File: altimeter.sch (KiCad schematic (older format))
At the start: 43 parts, among them Q101 DMG2301L, Q102 NTR4003NT1G, Q103 SISS05dn, U1 LMV331, U101 STM32F303CCTx, U102 S25FL512SAGMFIR11, U103 AIS2120SXTR, U104 MIC5219-3.3YM5, U105 LF50_TO252, U106 BMI088, U107 MS5611-01BA, Y1 Crystal_GND24

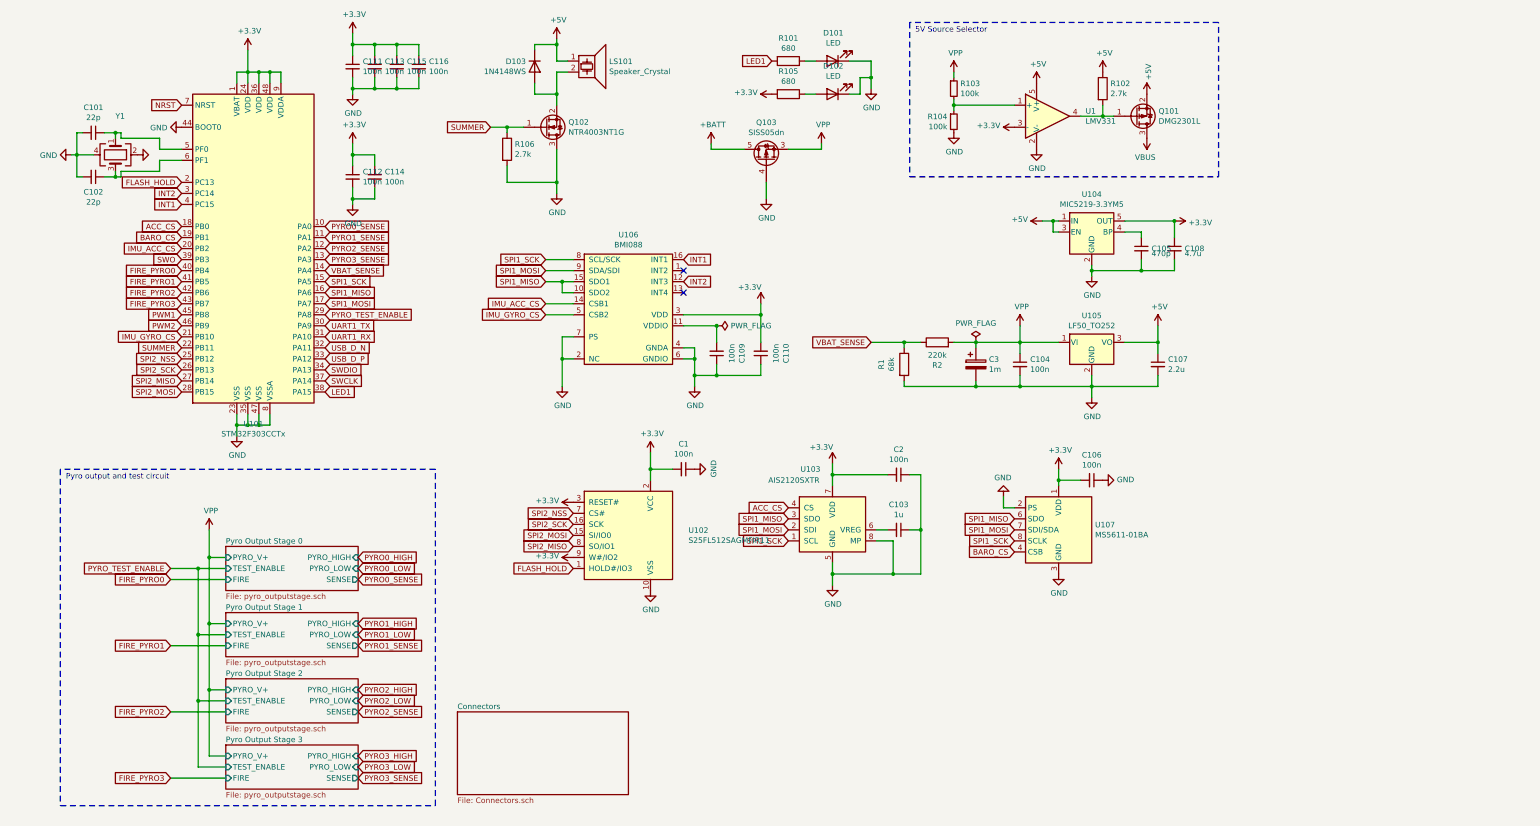
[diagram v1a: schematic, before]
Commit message: v1.2 rev A
Signed-off-by: Thomas Schmid <tom@binary-kitchen.de>
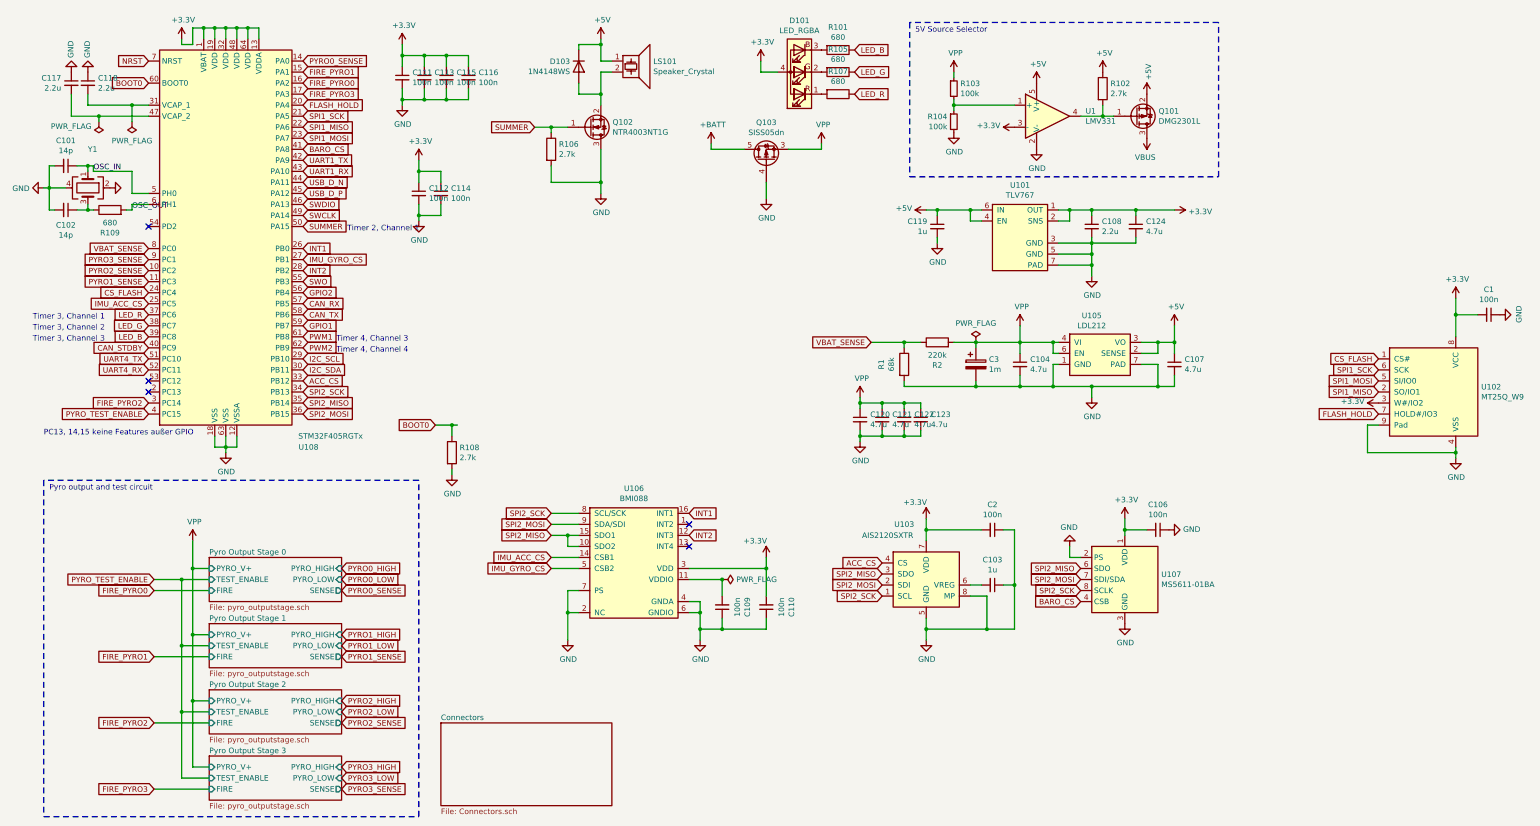
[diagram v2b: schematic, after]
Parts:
- removed C105: 470p, Capacitor_SMD:C_0603_1608Metric_Pad1.05x0.95mm_HandSolder, symbol Device:C_Small
- removed D101, D102: LED, LED_SMD:LED_0603_1608Metric, symbol Device:LED
- removed U101: STM32F303CCTx, Package_QFP:LQFP-48_7x7mm_P0.5mm, symbol MCU_ST_STM32F3:STM32F303CCTx
- removed U102: S25FL512SAGMFIR11, Package_SO:SOIC-16W_7.5x10.3mm_P1.27mm, symbol altimeter:S25L512S
- removed U104: MIC5219-3.3YM5, Package_TO_SOT_SMD:SOT-23-5, symbol Regulator_Linear:MIC5219-3.3YM5
- removed U105: LF50_TO252, Package_TO_SOT_SMD:TO-252-2, symbol Regulator_Linear:LF50_TO252
- added C117, C118: 2.2u, Capacitor_SMD:C_0402_1005Metric, symbol Device:C_Small
- added C119: 1u, Capacitor_SMD:C_0805_2012Metric, symbol Device:C_Small
- added C120, C121, C122, C123: 4.7u, Capacitor_SMD:C_0805_2012Metric_Pad1.15x1.40mm_HandSolder, symbol Device:C_Small
- added C124: 4.7u, Capacitor_SMD:C_0603_1608Metric_Pad1.05x0.95mm_HandSolder, symbol Device:C_Small
- added D101: LED_RGBA, altimeter:SMD_RGB_LED, symbol Device:LED_RGBA
- added R107, R109: 680, Resistor_SMD:R_0402_1005Metric, symbol Device:R
- added R108: 2.7k, Resistor_SMD:R_0402_1005Metric, symbol Device:R
- added U101: TLV767, altimeter:TI_WSON_TLV767, symbol altimeter:TLV767
- added U102: MT25Q_W9, altimeter:micron-wpdfn_8x6mm, symbol altimeter:MT25Q_W9
- added U105: LDL212, Package_DFN_QFN:DFN-6-1EP_3x3mm_P0.95mm_EP1.7x2.6mm, symbol altimeter:LDL212
- added U108: STM32F405RGTx, Package_QFP:LQFP-64_10x10mm_P0.5mm, symbol MCU_ST_STM32F4:STM32F405RGTx
- C101, C102: value 22p -> 14p
- C104: value 100n -> 4.7u
- C107: value 2.2u -> 4.7u; footprint Capacitor_SMD:C_0603_1608Metric_Pad1.05x0.95mm_HandSolder -> Capacitor_SMD:C_0805_2012Metric
- C108: value 4.7u -> 2.2u
- R106: Mouser_Link (none) -> https://www.mouser.de/ProductDetail/Vishay-Dale/CRCW04022K7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; Parnumber (none) -> CRCW04022K70FKEDC
- U1: footprint Package_TO_SOT_SMD:SOT-23-5 -> Package_TO_SOT_SMD:SOT-353_SC-70-5; Mouser_Link https://www.mouser.de/ProductDetail/ON-Semiconductor/LMV331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 -> https://www.mouser.de/datasheet/2/115/LMV331_393-335820.pdf; Parnumber LMV331SN3T1G -> LMV331SE-7
- Y1: footprint Crystal:Crystal_SMD_2520-4Pin_2.5x2.0mm -> Crystal:Crystal_SMD_2016-4Pin_2.0x1.6mm; Mouser_Link https://www.mouser.de/ProductDetail/Epson-Timing/TSX-3225-2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 -> https://www.mouser.de/ProductDetail/ECS/ECS-160-12-37B-CTN-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; Parnumber TSX-3225 24.0000MF15X-AC3 -> ECS-160-12-37B-CTN-TR
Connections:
- net +3V3: now also C124.1, D101.4 (A), U101.1 (OUT), U101.2 (SNS), U102.3 (W#/IO2), U102.8 (VCC), U108.1 (VBAT), U108.13 (VDDA), U108.19 (VDD), U108.32 (VDD), U108.48 (VDD), U108.64 (VDD); no longer R105.2
- net +5V: now also C119.1, U101.4 (EN), U101.6 (IN), U105.2 (SENSE), U105.3 (VO)
- net ACC_CS: now also U108.33 (PB12)
- net BARO_CS: now also U108.41 (PA8)
- net FIRE_PYRO0: now also U108.16 (PA2)
- net FIRE_PYRO1: now also U108.15 (PA1)
- net FIRE_PYRO2: now also U108.3 (PC14)
- net FIRE_PYRO3: now also U108.17 (PA3)
- net FLASH_HOLD: now also U102.7 (HOLD#/IO3), U108.20 (PA4)
- net GND: now also C117.1, C118.1, C119.2, C120.2, C121.2, C122.2, C123.2, C124.2, R108.2, U101.3 (GND), U101.5 (GND), U101.7 (PAD), U102.4 (VSS), U102.9 (Pad), U105.1 (GND), U105.7 (PAD), U108.12 (VSSA), U108.18 (VSS), U108.63 (VSS)
- net IMU_ACC_CS: now also U108.25 (PC5)
- net IMU_GYRO_CS: now also U108.27 (PB1)
- net INT1: now also U108.26 (PB0)
- net INT2: now also U108.28 (PB2)
- net NRST: now also U108.7 (NRST)
- net PWM1: now also U108.61 (PB8)
- net PWM2: now also U108.62 (PB9)
- net PYRO0_SENSE: now also U108.14 (PA0)
- net PYRO1_SENSE: now also U108.11 (PC3)
- net PYRO2_SENSE: now also U108.10 (PC2)
- net PYRO3_SENSE: now also U108.9 (PC1)
- net PYRO_TEST_ENABLE: now also U108.4 (PC15)
- net SPI1_MISO: now also U102.2 (SO/IO1), U108.22 (PA6); no longer U103.3 (SDO), U106.10 (SDO2), U106.15 (SDO1), U107.6 (SDO)
- net SPI1_MOSI: now also U102.5 (SI/IO0), U108.23 (PA7); no longer U103.2 (SDI), U106.9 (SDA/SDI), U107.7 (SDI/SDA)
- net SPI1_SCK: now also U102.6 (SCK), U108.21 (PA5); no longer U103.1 (SCL), U106.8 (SCL/SCK), U107.8 (SCLK)
- net SPI2_MISO: now also U103.3 (SDO), U106.10 (SDO2), U106.15 (SDO1), U107.6 (SDO), U108.35 (PB14)
- net SPI2_MOSI: now also U103.2 (SDI), U106.9 (SDA/SDI), U107.7 (SDI/SDA), U108.36 (PB15)
- net SPI2_SCK: now also U103.1 (SCL), U106.8 (SCL/SCK), U107.8 (SCLK), U108.34 (PB13)
- net SUMMER: now also U108.50 (PA15)
- net SWCLK: now also U108.49 (PA14)
- net SWDIO: now also U108.46 (PA13)
- net SWO: now also U108.55 (PB3)
- net UART1_RX: now also U108.43 (PA10)
- net UART1_TX: now also U108.42 (PA9)
- net USB_D_N: now also U108.44 (PA11)
- net USB_D_P: now also U108.45 (PA12)
- net VBAT_SENSE: now also U108.8 (PC0)
- net VPP: now also C120.1, C121.1, C122.1, C123.1, U105.4 (VI), U105.6 (EN)
- net OSC_IN: now reaches C101.1, Y1.1
- net OSC_IN: now also U108.5 (PH0)
- net at C102.1, Y1.3: now also R109.1
- net LED_B: now reaches R101.1
- net LED_B: now also U108.39 (PC8)
- net LED_G: now reaches R105.1
- net LED_G: now also U108.38 (PC7)
- net LED1: no longer names the net of R101.2
- net LED1: now also D101.3 (BK)
- new net: C118.2, U108.31 (VCAP_1)
- new net: C117.2, U108.47 (VCAP_2)
- new net: D101.1 (RK), R107.2
- new net: D101.2 (GK), R105.2
- new net BOOT0: R108.1, U108.60 (BOOT0)
- new net CAN_RX: U108.57 (PB5)
- new net CAN_STDBY: U108.40 (PC9)
- new net CAN_TX: U108.58 (PB6)
- new net CS_FLASH: U102.1 (CS#), U108.24 (PC4)
- new net GPIO1: U108.59 (PB7)
- new net GPIO2: U108.56 (PB4)
- new net I2C_SCL: U108.29 (PB10)
- new net I2C_SDA: U108.30 (PB11)
- new net LED_R: R107.1, U108.37 (PC6)
- new net OSC_OUT: R109.2, U108.6 (PH1)
- new net UART4_RX: U108.52 (PC11)
- new net UART4_TX: U108.51 (PC10)
- no-connect marks 2 -> 5
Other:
- note added: "PC13, 14,15 keine Features außer GPIO\n"
- note added: "Timer 2, Channel 1"
- note added: "Timer 3, Channel 1"
- note added: "Timer 3, Channel 2"
- note added: "Timer 3, Channel 3"
- note added: "Timer 4, Channel 3"
- note added: "Timer 4, Channel 4"
- moved on the sheet: C1, C101, C102, C103, C106, C107, C108, C109, C110, C111, C112, C113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

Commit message: update
Signed-off-by: Thomas Schmid <tom@binary-kitchen.de>
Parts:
- C104, C120, C121, C122, C123: Mouser_Link https://www.mouser.de/ProductDetail/KEMET/C0805C104Z3VACTU?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 -> https://www.mouser.de/ProductDetail/Taiyo-Yuden/GMK212BBJ47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; Parnumber C0805C104Z3VACTU -> GMK212BBJ475KD-T
- C107: Mouser_Link https://www.mouser.de/ProductDetail/Taiyo-Yuden/EMK107BJ225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 -> https://www.mouser.de/ProductDetail/Taiyo-Yuden/GMK212BBJ47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; Parnumber EMK107BJ225MA-T -> GMK212BBJ475KD-T
- C108: Mouser_Link https://www.mouser.de/ProductDetail/Taiyo-Yuden/EMK107ABJ47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 -> (none); Parnumber EMK107ABJ475KA-T -> EMK107BJ225MA-T
- C117, C118: Mouser_Link https://www.mouser.de/ProductDetail/Wurth-Elektronik/885012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 -> https://www.mouser.de/ProductDetail/Yageo/CC0402KRX5R7BB225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; Parnumber 885012205037 -> CC0402KRX5R7BB225
- C119: Mouser_Link https://www.mouser.de/ProductDetail/Taiyo-Yuden/EMK107BJ225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 -> https://www.mouser.de/ProductDetail/Taiyo-Yuden/UMF212B7105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; Parnumber EMK107BJ225MA-T -> UMF212B7105KGHT
- C124: Mouser_Link https://www.mouser.de/ProductDetail/Taiyo-Yuden/EMK107ABJ47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 -> https://www.mouser.de/ProductDetail/Murata-Electronics/GRM1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; Parnumber EMK107ABJ475KA-T -> GRM188R60J475KE19D
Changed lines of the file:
@@
 F 2 "Capacitor_SMD:C_0805_2012Metric_Pad1.15x1.40mm_HandSolder" H 9350 3650 50  0001 C CNN
 F 3 "~" H 9350 3650 50  0001 C CNN
-F 4 "https://www.mouser.de/ProductDetail/KEMET/C0805C104Z3VACTU?qs=sGAEpiMZZMs0AnBnWHyRQFCCI5cSbRT%2FdZzrd8bbt%252Bc%3D" H 9350 3650 50  0001 C CNN "Mouser_Link"
-F 5 "C0805C104Z3VACTU" H 9350 3650 50  0001 C CNN "Parnumber"
+F 4 "https://www.mouser.de/ProductDetail/Taiyo-Yuden/GMK212BBJ475KD-T?qs=VWNNG7jHlrJu0gRQmF8TjA%3D%3D" H 9350 3650 50  0001 C CNN "Mouser_Link"
+F 5 "GMK212BBJ475KD-T" H 9350 3650 50  0001 C CNN "Parnumber"
 	1    9350 3650
 	1    0    0    -1
@@
 F 2 "Capacitor_SMD:C_0805_2012Metric" H 10750 3650 50  0001 C CNN
 F 3 "~" H 10750 3650 50  0001 C CNN
-F 4 "https://www.mouser.de/ProductDetail/Taiyo-Yuden/EMK107BJ225MA-T?qs=sGAEpiMZZMs0AnBnWHyRQPSjYu%2Fkbgu8gi8YbsqojVfHLlKjG2ASkw%3D%3D" H 10750 3650 50  0001 C CNN "Mouser_Link"
-F 5 "EMK107BJ225MA-T" H 10750 3650 50  0001 C CNN "Parnumber"
+F 4 "https://www.mouser.de/ProductDetail/Taiyo-Yuden/GMK212BBJ475KD-T?qs=VWNNG7jHlrJu0gRQmF8TjA%3D%3D" H 10750 3650 50  0001 C CNN "Mouser_Link"
+F 5 "GMK212BBJ475KD-T" H 10750 3650 50  0001 C CNN "Parnumber"
 	1    10750 3650
 	1    0    0    -1
@@
 F 2 "Capacitor_SMD:C_0603_1608Metric_Pad1.05x0.95mm_HandSolder" H 10000 2400 50  0001 C CNN
 F 3 "~" H 10000 2400 50  0001 C CNN
-F 4 "https://www.mouser.de/ProductDetail/Taiyo-Yuden/EMK107ABJ475KA-T?qs=sGAEpiMZZMsh%252B1woXyUXjzXZPAgA2%252BEM0YjaF6PuMqo%3D" H 10000 2400 50  0001 C CNN "Mouser_Link"
-F 5 "EMK107ABJ475KA-T" H 10000 2400 50  0001 C CNN "Parnumber"
+F 4 "" H 10000 2400 50  0001 C CNN "Mouser_Link"
+F 5 "EMK107BJ225MA-T" H 10000 2400 50  0001 C CNN "Parnumber"
 	1    10000 2400
 	1    0    0    -1
@@
 F 2 "Capacitor_SMD:C_0402_1005Metric" H 900 1100 50  0001 C CNN
 F 3 "~" H 900 1100 50  0001 C CNN
-F 4 "https://www.mouser.de/ProductDetail/Wurth-Elektronik/885012205037?qs=sGAEpiMZZMs0AnBnWHyRQEGbLOF2VP1iQ21DRO%252BfKQRXXkG1Pup5LQ%3D%3D" H 900 1100 50  0001 C CNN "Mouser_Link"
-F 5 "885012205037" H 900 1100 50  0001 C CNN "Parnumber"
+F 4 "https://www.mouser.de/ProductDetail/Yageo/CC0402KRX5R7BB225?qs=shS2SvXCj6KxdMpn6SQPQQ%3D%3D" H 900 1100 50  0001 C CNN "Mouser_Link"
+F 5 "CC0402KRX5R7BB225 " H 900 1100 50  0001 C CNN "Parnumber"
 	1    900  1100
 	1    0    0    -1
@@
 F 2 "Capacitor_SMD:C_0402_1005Metric" H 750 1100 50  0001 C CNN
 F 3 "~" H 750 1100 50  0001 C CNN
-F 4 "https://www.mouser.de/ProductDetail/Wurth-Elektronik/885012205037?qs=sGAEpiMZZMs0AnBnWHyRQEGbLOF2VP1iQ21DRO%252BfKQRXXkG1Pup5LQ%3D%3D" H 750 1100 50  0001 C CNN "Mouser_Link"
-F 5 "885012205037" H 750 1100 50  0001 C CNN "Parnumber"
+F 4 "https://www.mouser.de/ProductDetail/Yageo/CC0402KRX5R7BB225?qs=shS2SvXCj6KxdMpn6SQPQQ%3D%3D" H 750 1100 50  0001 C CNN "Mouser_Link"
+F 5 "CC0402KRX5R7BB225 " H 750 1100 50  0001 C CNN "Parnumber"
 	1    750  1100
 	1    0    0    -1
@@
 F 2 "Capacitor_SMD:C_0805_2012Metric" H 8600 2400 50  0001 C CNN
 F 3 "~" H 8600 2400 50  0001 C CNN
-F 4 "https://www.mouser.de/ProductDetail/Taiyo-Yuden/EMK107BJ225MA-T?qs=sGAEpiMZZMs0AnBnWHyRQPSjYu%2Fkbgu8gi8YbsqojVfHLlKjG2ASkw%3D%3D" H 8600 2400 50  0001 C CNN "Mouser_Link"
-F 5 "EMK107BJ225MA-T" H 8600 2400 50  0001 C CNN "Parnumber"
+F 4 "https://www.mouser.de/ProductDetail/Taiyo-Yuden/UMF212B7105KGHT?qs=%252B6g0mu59x7KoF6NN%2FES6FQ%3D%3D" H 8600 2400 50  0001 C CNN "Mouser_Link"
+F 5 "UMF212B7105KGHT" H 8600 2400 50  0001 C CNN "Parnumber"
 	1    8600 2400
 	1    0    0    -1
@@
 F 2 "Capacitor_SMD:C_0805_2012Metric_Pad1.15x1.40mm_HandSolder" H 7900 4150 50  0001 C CNN
 F 3 "~" H 7900 4150 50  0001 C CNN
-F 4 "https://www.mouser.de/ProductDetail/KEMET/C0805C104Z3VACTU?qs=sGAEpiMZZMs0AnBnWHyRQFCCI5cSbRT%2FdZzrd8bbt%252Bc%3D" H 7900 4150 50  0001 C CNN "Mouser_Link"
-F 5 "C0805C104Z3VACTU" H 7900 4150 50  0001 C CNN "Parnumber"
+F 4 "https://www.mouser.de/ProductDetail/Taiyo-Yuden/GMK212BBJ475KD-T?qs=VWNNG7jHlrJu0gRQmF8TjA%3D%3D" H 7900 4150 50  0001 C CNN "Mouser_Link"
+F 5 "GMK212BBJ475KD-T" H 7900 4150 50  0001 C CNN "Parnumber"
 	1    7900 4150
 	1    0    0    -1
@@
 F 2 "Capacitor_SMD:C_0805_2012Metric_Pad1.15x1.40mm_HandSolder" H 8100 4150 50  0001 C CNN
 F 3 "~" H 8100 4150 50  0001 C CNN
-F 4 "https://www.mouser.de/ProductDetail/KEMET/C0805C104Z3VACTU?qs=sGAEpiMZZMs0AnBnWHyRQFCCI5cSbRT%2FdZzrd8bbt%252Bc%3D" H 8100 4150 50  0001 C CNN "Mouser_Link"
-F 5 "C0805C104Z3VACTU" H 8100 4150 50  0001 C CNN "Parnumber"
+F 4 "https://www.mouser.de/ProductDetail/Taiyo-Yuden/GMK212BBJ475KD-T?qs=VWNNG7jHlrJu0gRQmF8TjA%3D%3D" H 8100 4150 50  0001 C CNN "Mouser_Link"
+F 5 "GMK212BBJ475KD-T" H 8100 4150 50  0001 C CNN "Parnumber"
 	1    8100 4150
 	1    0    0    -1
@@
 F 2 "Capacitor_SMD:C_0805_2012Metric_Pad1.15x1.40mm_HandSolder" H 8300 4150 50  0001 C CNN
 F 3 "~" H 8300 4150 50  0001 C CNN
-F 4 "https://www.mouser.de/ProductDetail/KEMET/C0805C104Z3VACTU?qs=sGAEpiMZZMs0AnBnWHyRQFCCI5cSbRT%2FdZzrd8bbt%252Bc%3D" H 8300 4150 50  0001 C CNN "Mouser_Link"
-F 5 "C0805C104Z3VACTU" H 8300 4150 50  0001 C CNN "Parnumber"
+F 4 "https://www.mouser.de/ProductDetail/Taiyo-Yuden/GMK212BBJ475KD-T?qs=VWNNG7jHlrJu0gRQmF8TjA%3D%3D" H 8300 4150 50  0001 C CNN "Mouser_Link"
+F 5 "GMK212BBJ475KD-T" H 8300 4150 50  0001 C CNN "Parnumber"
 	1    8300 4150
 	1    0    0    -1
@@
 F 2 "Capacitor_SMD:C_0805_2012Metric_Pad1.15x1.40mm_HandSolder" H 8450 4150 50  0001 C CNN
 F 3 "~" H 8450 4150 50  0001 C CNN
-F 4 "https://www.mouser.de/ProductDetail/KEMET/C0805C104Z3VACTU?qs=sGAEpiMZZMs0AnBnWHyRQFCCI5cSbRT%2FdZzrd8bbt%252Bc%3D" H 8450 4150 50  0001 C CNN "Mouser_Link"
-F 5 "C0805C104Z3VACTU" H 8450 4150 50  0001 C CNN "Parnumber"
+F 4 "https://www.mouser.de/ProductDetail/Taiyo-Yuden/GMK212BBJ475KD-T?qs=VWNNG7jHlrJu0gRQmF8TjA%3D%3D" H 8450 4150 50  0001 C CNN "Mouser_Link"
+F 5 "GMK212BBJ475KD-T" H 8450 4150 50  0001 C CNN "Parnumber"
 	1    8450 4150
 	1    0    0    -1
@@
 F 2 "Capacitor_SMD:C_0603_1608Metric_Pad1.05x0.95mm_HandSolder" H 10400 2400 50  0001 C CNN
 F 3 "~" H 10400 2400 50  0001 C CNN
-F 4 "https://www.mouser.de/ProductDetail/Taiyo-Yuden/EMK107ABJ475KA-T?qs=sGAEpiMZZMsh%252B1woXyUXjzXZPAgA2%252BEM0YjaF6PuMqo%3D" H 10400 2400 50  0001 C CNN "Mouser_Link"
-F 5 "EMK107ABJ475KA-T" H 10400 2400 50  0001 C CNN "Parnumber"
+F 4 "https://www.mouser.de/ProductDetail/Murata-Electronics/GRM188R60J475KE19D?qs=8N7GLiuM2OS81roWI9UfgQ%3D%3D" H 10400 2400 50  0001 C CNN "Mouser_Link"
+F 5 "GRM188R60J475KE19D " H 10400 2400 50  0001 C CNN "Parnumber"
 	1    10400 2400
 	1    0    0    -1
